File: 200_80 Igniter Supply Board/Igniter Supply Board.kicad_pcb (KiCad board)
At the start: 4 copper layers, 80 x 49 mm, 91 parts, among them J1 BNC, J2 BNC, J3 53261-1371, Q1 G2R1000MT33J-TR, Q2 BSS123, Q3 BSS123, Q4 BSS123, Q5 BSS123, T1 750319697, U1 OP37, U2 OP37, U3 OP37, U4 LMP2022, U5 LT8301, U7 Si8261BAC

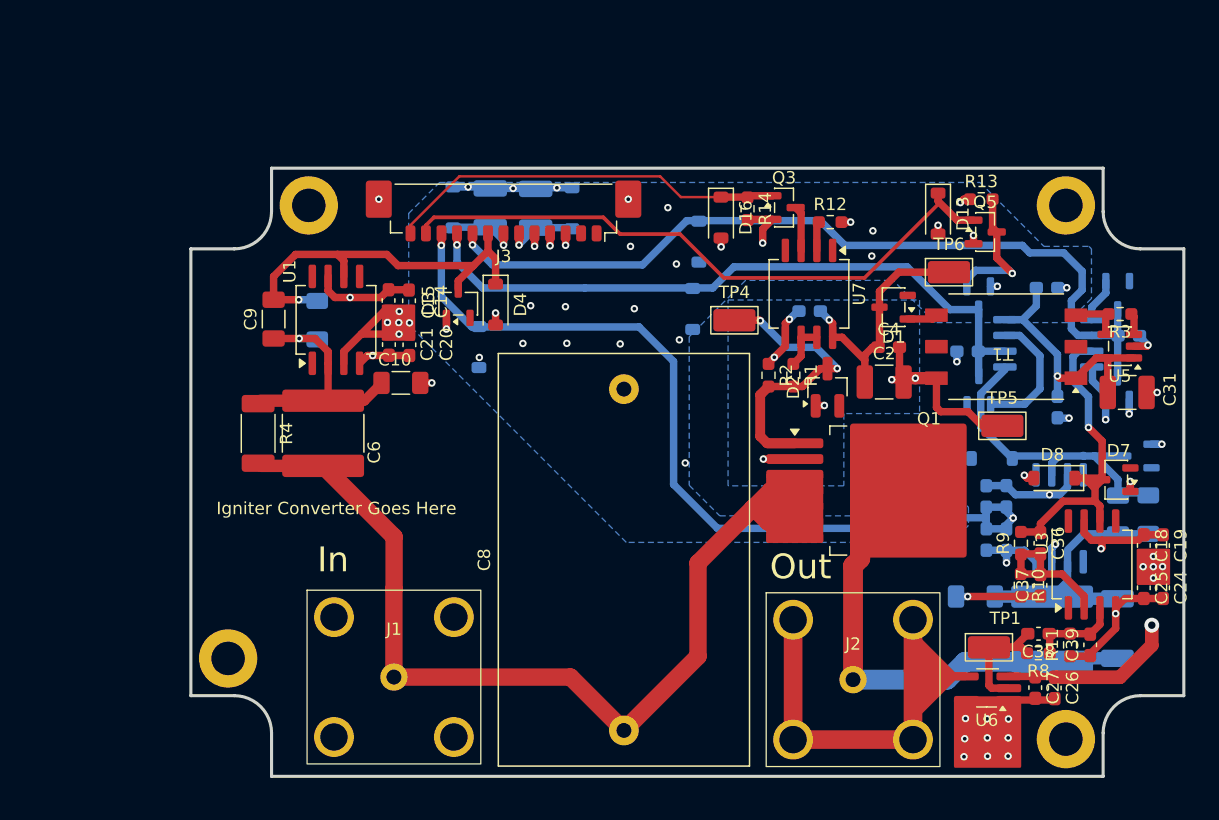
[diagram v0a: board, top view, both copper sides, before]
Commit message: Igniter board + discharge board first final draft
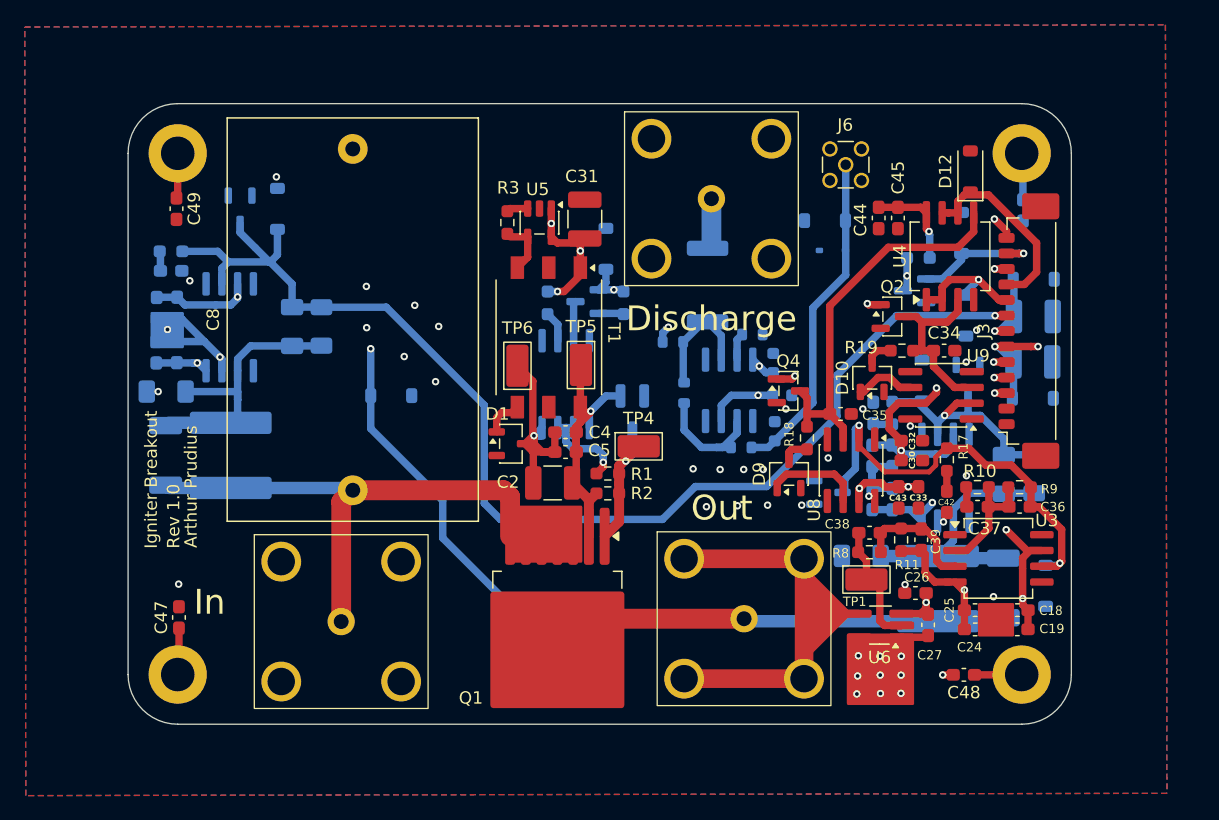
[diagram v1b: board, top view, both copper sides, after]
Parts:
- removed ? (x3): , 
- added C1: 100n, Capacitor_SMD:C_0603_1608Metric, B.Cu at (140.7, 101.5)
- added C3: 100n, Capacitor_SMD:C_0603_1608Metric, B.Cu at (140.0, 98.9)
- added C33: 100nF, Capacitor_SMD:C_0603_1608Metric_Pad1.08x0.95mm_HandSolder, F.Cu at (151.7, 109.7)
- added C40: 500pF, Capacitor_SMD:C_0603_1608Metric_Pad1.08x0.95mm_HandSolder, B.Cu at (91.5, 91.5)
- added C41: 500pF, Capacitor_SMD:C_0603_1608Metric_Pad1.08x0.95mm_HandSolder, B.Cu at (148.0, 102.9)
- added C42: 500pF, Capacitor_SMD:C_0603_1608Metric_Pad1.08x0.95mm_HandSolder, F.Cu at (154.0, 110.1)
- added C43: 1nF, Capacitor_SMD:C_0603_1608Metric_Pad1.08x0.95mm_HandSolder, F.Cu at (150.1, 109.7)
- added C44: 100nF, Capacitor_SMD:C_0603_1608Metric_Pad1.08x0.95mm_HandSolder, F.Cu at (148.5, 87.2)
- added C45: 1nF, Capacitor_SMD:C_0603_1608Metric_Pad1.08x0.95mm_HandSolder, F.Cu at (150.0, 87.2)
- added C46: 100nF, Capacitor_SMD:C_0603_1608Metric_Pad1.08x0.95mm_HandSolder, B.Cu at (160.1, 86.6)
- added C47: 100nF, Capacitor_SMD:C_0603_1608Metric_Pad1.08x0.95mm_HandSolder, F.Cu at (92.1, 119.4)
- added C48: 100nF, Capacitor_SMD:C_0603_1608Metric_Pad1.08x0.95mm_HandSolder, F.Cu at (155.3, 124.0)
- added C49: 100nF, Capacitor_SMD:C_0603_1608Metric_Pad1.08x0.95mm_HandSolder, F.Cu at (91.9, 86.5)
- added C51: 100n, Capacitor_SMD:C_0603_1608Metric, B.Cu at (140.1, 104.4)
- added D18: BAT54WS, Diode_SMD:D_SOD-323, B.Cu at (144.8, 89.8)
- added D19: MMSZ4685, Diode_SMD:D_SOD-123, B.Cu at (144.2, 87.4)
- added H1: M2.5, MountingHole:MountingHole_2.7mm_M2.5_DIN965_Pad, F.Cu at (160.0, 82.0)
- added H2: M2.5, MountingHole:MountingHole_2.7mm_M2.5_DIN965_Pad, F.Cu at (92.0, 124.0)
- added H4: M2.5, MountingHole:MountingHole_2.7mm_M2.5_DIN965_Pad, F.Cu at (92.0, 82.0)
- added J4: 112659, 0_PAY_Footprint_Library:CONN_112659, F.Cu at (135.0, 85.7)
- added J6: MMCX, Connector_Coaxial:MMCX_Molex_73415-1471_Vertical, F.Cu at (145.8, 82.9)
- added R15: 50R, Resistor_SMD:R_0603_1608Metric_Pad0.98x0.95mm_HandSolder, B.Cu at (91.5, 89.9)
- added R16: 50R, Resistor_SMD:R_0603_1608Metric_Pad0.98x0.95mm_HandSolder, B.Cu at (149.6, 102.9)
- added R17: 50R, Resistor_SMD:R_0603_1608Metric_Pad0.98x0.95mm_HandSolder, F.Cu at (154.0, 106.7)
- added R18: 100R, Resistor_SMD:R_0603_1608Metric_Pad0.98x0.95mm_HandSolder, F.Cu at (142.7, 104.9)
- added R19: 100R, Resistor_SMD:R_0603_1608Metric_Pad0.98x0.95mm_HandSolder, F.Cu at (150.3, 97.9)
- added R20: 4M 1%, Resistor_SMD:R_2512_6332Metric, B.Cu at (134.7, 92.6)
- added R21: 4.53k 1%, Resistor_SMD:R_0603_1608Metric, B.Cu at (131.9, 97.2)
- added R22: 3.74k 1%, Resistor_SMD:R_0603_1608Metric, B.Cu at (138.3, 96.6)
- added R23: 22.6k 0.1%, Resistor_SMD:R_0603_1608Metric, B.Cu at (132.8, 101.3)
- added R24: 100, Resistor_SMD:R_0603_1608Metric, B.Cu at (137.4, 105.7)
- added U10: OP37, Package_SO:SOIC-8_3.9x4.9mm_P1.27mm, B.Cu at (136.4, 101.1)
- added U8: MAX997ESA, Package_SO:SOIC-8_3.9x4.9mm_P1.27mm, F.Cu at (146.2, 107.5)
- added U9: MAX997ESA, Package_SO:SOIC-8_3.9x4.9mm_P1.27mm, F.Cu at (153.5, 101.5)
- C10, C14, C15, C20, C21, C6, C9, D13, D16, D2, D3, D4, D7, D8, Q3, Q5, R12, R13, R14, R4, U1, U7: moved to B.Cu
- C30, C32, C34, C35, C5, D10, D12, D9, Q2, Q4: moved to F.Cu
- U4: value LMP2022 -> LMP2022MM; moved to F.Cu
- moved H3 64.0 mm to (160.0, 124.0)
- moved R3 49.9 mm to (118.6, 87.6), turned to -90 degrees
- moved U5 47.8 mm to (121.1, 87.6), turned to -90 degrees
- moved D14 47.1 mm to (161.0, 92.2), turned to 0 degrees
- moved C31 45.9 mm to (124.8, 87.3), turned to 90 degrees
- moved C28 44.6 mm to (160.9, 95.2), turned to 0 degrees
- moved J3 42.8 mm to (160.0, 96.3), turned to 90 degrees
- moved C29 41.9 mm to (160.9, 98.8), turned to 180 degrees
- moved D15 40.2 mm to (160.9, 101.7), turned to 180 degrees
- moved T1 36.5 mm to (122.0, 97.1), turned to -90 degrees
- moved TP6 35.6 mm to (119.4, 99.1), turned to 90 degrees
- moved TP5 34.3 mm to (124.5, 99.1), turned to -90 degrees
- moved D1 32.7 mm to (118.8, 105.4), turned to 0 degrees
- moved TH1 31.3 mm to (122.5, 121.8)
- moved D9 30.1 mm to (141.2, 107.8), turned to 90 degrees
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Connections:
- C34 pad 1: /ADC_V_IGN_PK -> Net-(Q2-D)
- C35 pad 1: /ADC_I_IGN_PK -> Net-(Q4-D)
- D10 pad 3: /ADC_V_IGN_PK -> Net-(D10-K)
- D9 pad 3: /ADC_I_IGN_PK -> Net-(D9-K)
- J3 pad 10: /ADC_V_IGN_PK -> /ADC_I_IGN_PK
- J3 pad 9: /ADC_I_IGN_PK -> /ADC_V_IGN_PK
- Q2 pad 3: /ADC_V_IGN_PK -> Net-(Q2-D)
- Q4 pad 3: /ADC_I_IGN_PK -> Net-(Q4-D)
- U4 pad 1: Net-(D9-A) -> /ADC_V_IGN_PK
- U4 pad 2: /ADC_I_IGN_PK -> /ADC_V_IGN_PK
- U4 pad 3: Net-(D7-K) -> Net-(Q2-D)
- U4 pad 5: Net-(D5-K) -> Net-(Q4-D)
- U4 pad 6: /ADC_V_IGN_PK -> /ADC_I_IGN_PK
- U4 pad 7: Net-(D10-A) -> /ADC_I_IGN_PK
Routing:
- net /ADC_V_IGN_SUPPLY: track 33.1 -> 98.8 mm
- net /ADC_I_IGN_PK: track 68.3 -> 15.5 mm, vias 1 -> 0
- net /ADC_V_IGN_PK: track 54.9 -> 10.1 mm
- net /IGNITER_RST: track 51.7 -> 10.6 mm, vias 0 -> 1
- net GND: track 82.7 -> 43.0 mm, vias 61 -> 45
- net Net-(J1-In): track 78.4 -> 42.3 mm
- net -5V: track 25.9 -> 58.4 mm, vias 4 -> 6
- net Net-(Q4-D): track 0.00 -> 31.8 mm
- net /ADC_NTC_IGN: track 56.9 -> 84.9 mm, vias 1 -> 2
- net /Discharge/DISCHARGE_V: track 0.00 -> 26.7 mm
- net 5V: track 68.1 -> 86.6 mm, vias 8 -> 14
- net Net-(Q2-D): track 0.00 -> 14.8 mm
- net Net-(D2-K): track 23.3 -> 10.9 mm, vias 2 -> 1
- net /IGNITER_nRST: track 27.6 -> 17.8 mm, vias 2 -> 3
- net /Discharge/AMP_OUT: track 0.00 -> 9.65 mm
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- added copper zone on F.Cu, net GND
- removed copper zone on B.Cu, net Net-(D2-A)
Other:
- board size 80 x 49 mm -> 76 x 50 mm
- board text added: "Discharge"
- board text removed: "Igniter Converter Goes Here"
